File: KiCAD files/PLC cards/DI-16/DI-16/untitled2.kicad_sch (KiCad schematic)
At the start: 28 parts

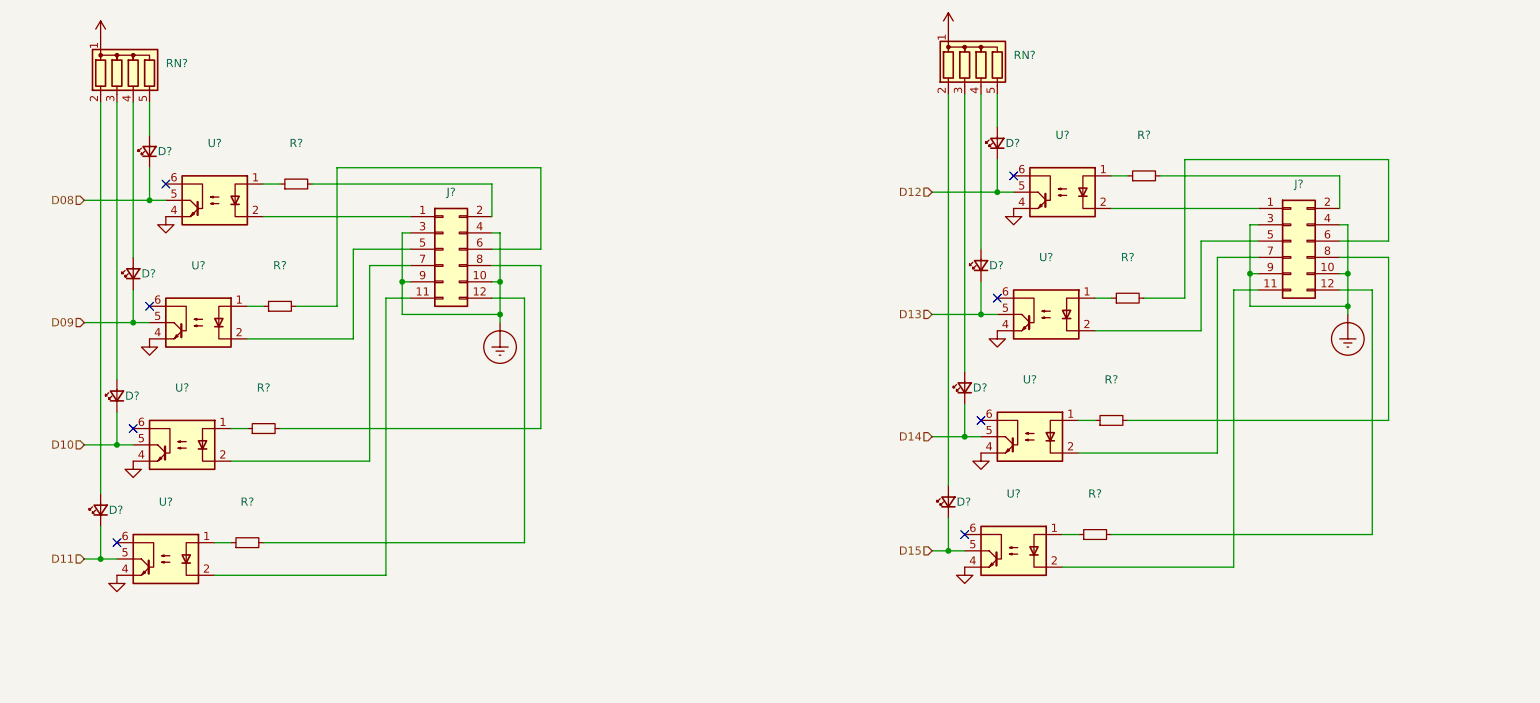
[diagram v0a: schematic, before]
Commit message: pcbs
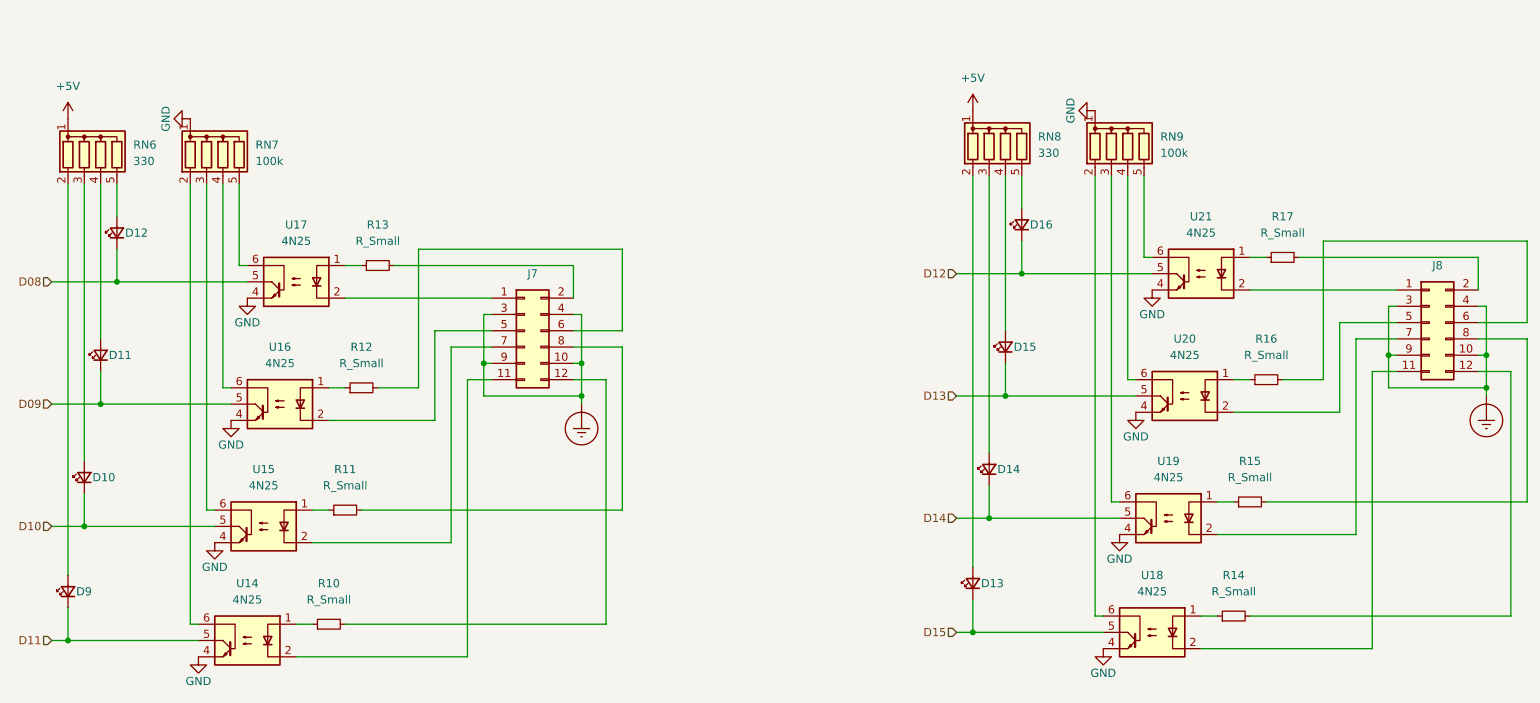
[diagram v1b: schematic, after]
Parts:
- removed D? (x8): (no value), symbol Device:LED_Small
- removed J? (x2): (no value), symbol Connector_Generic:Conn_02x06_Odd_Even
- removed R? (x8): (no value), symbol Device:R_Small
- removed RN? (x2): (no value), symbol Device:R_Network04
- removed U? (x8): (no value), symbol Isolator:4N25
- added D10, D11, D12, D13, D14, D15, D16, D9: LED_Small, symbol Device:LED_Small
- added J7, J8: Conn_02x06_Odd_Even, symbol Connector_Generic:Conn_02x06_Odd_Even
- added R10, R11, R12, R13, R14, R15, R16, R17: R_Small, symbol Device:R_Small
- added RN6, RN8: 330, Resistor_THT:R_Array_SIP5, symbol Device:R_Network04
- added RN7, RN9: 100k, Resistor_THT:R_Array_SIP5, symbol Device:R_Network04
- added U14, U15, U16, U17, U18, U19, U20, U21: 4N25, Package_DIP:DIP-6_W7.62mm, symbol Isolator:4N25
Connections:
- net +5V: now also RN6.1 (common), RN8.1 (common)
- net D08: now also D12.1 (K), U17.5
- net D09: now also D11.1 (K), U16.5
- net D10: now also D10.1 (K), U15.5
- net D11: now also D9.1 (K), U14.5
- net D12: now also D16.1 (K), U21.5
- net D13: now also D15.1 (K), U20.5
- net D14: now also D14.1 (K), U19.5
- net D15: now also D13.1 (K), U18.5
- net Earth_Protective: now also J7.10 (Pin_10), J7.3 (Pin_3), J7.4 (Pin_4), J7.9 (Pin_9), J8.10 (Pin_10), J8.3 (Pin_3), J8.4 (Pin_4), J8.9 (Pin_9)
- net GND: now also RN7.1 (common), RN9.1 (common), U14.4, U15.4, U16.4, U17.4, U18.4, U19.4, U20.4, U21.4
- new net: R16.1, U20.1
- new net: J8.6 (Pin_6), R16.2
- new net: R10.1, U14.1
- new net: J7.12 (Pin_12), R10.2
- new net: D14.2 (A), RN8.3 (R2)
- new net: R11.1, U15.1
- new net: J7.7 (Pin_7), U15.2
- new net: RN7.3 (R2), U15.6
- new net: R17.1, U21.1
- new net: J8.2 (Pin_2), R17.2
- new net: R12.1, U16.1
- new net: J7.5 (Pin_5), U16.2
- new net: RN7.4 (R3), U16.6
- new net: J7.1 (Pin_1), U17.2
- new net: J7.11 (Pin_11), U14.2
- new net: J7.2 (Pin_2), R13.2
- new net: J7.6 (Pin_6), R12.2
- new net: J7.8 (Pin_8), R11.2
- new net: D10.2 (A), RN6.3 (R2)
- new net: R14.1, U18.1
- new net: J8.12 (Pin_12), R14.2
- new net: J8.1 (Pin_1), U21.2
- new net: J8.11 (Pin_11), U18.2
- new net: J8.5 (Pin_5), U20.2
- new net: J8.7 (Pin_7), U19.2
- new net: J8.8 (Pin_8), R15.2
- new net: RN9.2 (R1), U18.6
- new net: RN9.4 (R3), U20.6
- new net: D9.2 (A), RN6.2 (R1)
- new net: D11.2 (A), RN6.4 (R3)
- new net: D12.2 (A), RN6.5 (R4)
- new net: RN7.2 (R1), U14.6
- new net: RN9.3 (R2), U19.6
- new net: RN9.5 (R4), U21.6
- new net: D15.2 (A), RN8.4 (R3)
- new net: D13.2 (A), RN8.2 (R1)
- new net: D16.2 (A), RN8.5 (R4)
- new net: R15.1, U19.1
- new net: RN7.5 (R4), U17.6
- new net: R13.1, U17.1
- no-connect marks 8 -> 0
